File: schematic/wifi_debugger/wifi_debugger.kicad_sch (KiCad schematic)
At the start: 4 parts, among them J1 USB4500-03-0-A_REVA, U1 ESP32-S3-WROOM-1

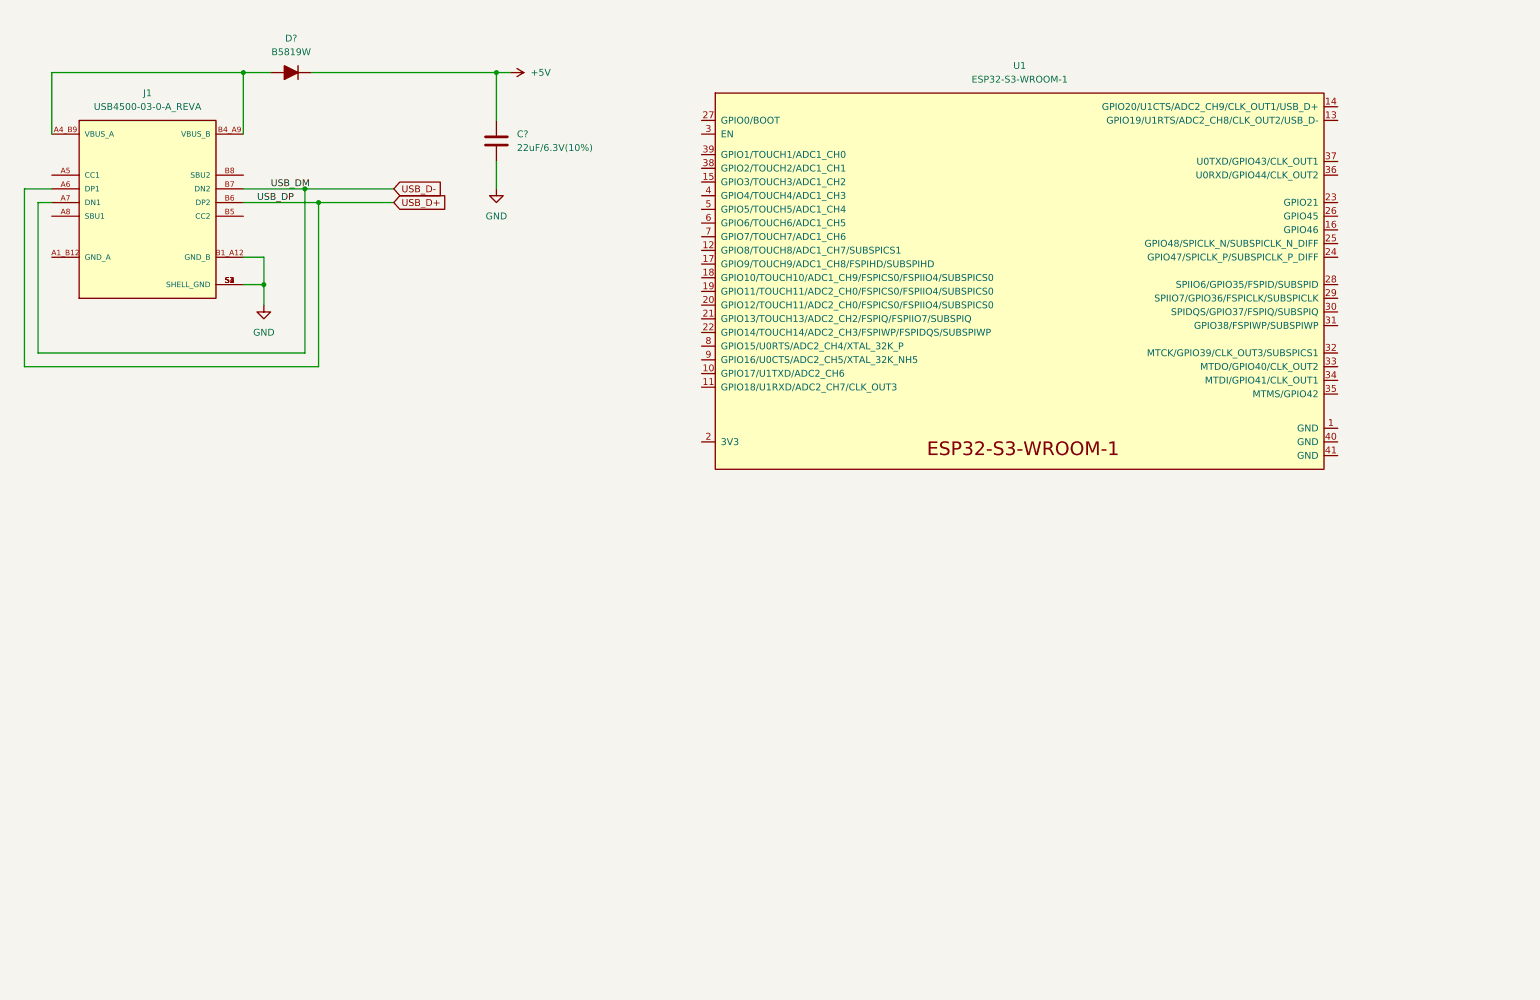
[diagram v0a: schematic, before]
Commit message: update
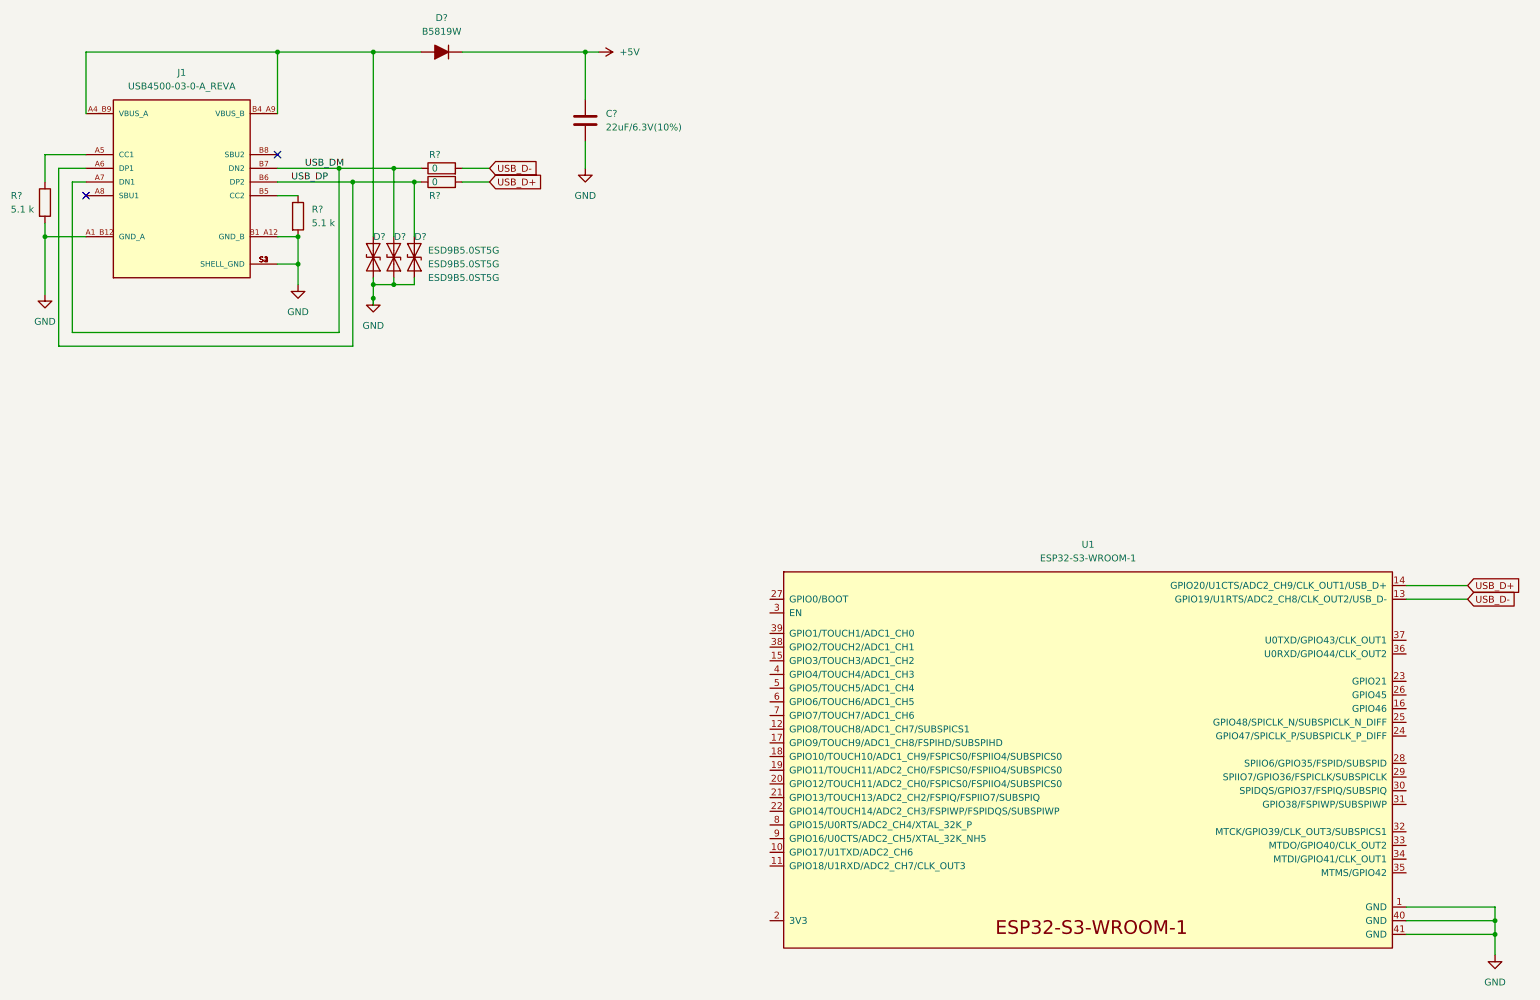
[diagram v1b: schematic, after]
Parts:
- added D? (x3): ESD9B5.0ST5G, Diode_SMD:D_SOD-923, symbol Diode:ESD9B5.0ST5G
- added R? (x2): 5.1 k, symbol Device:R
- added R? (x2): 0, symbol Device:R
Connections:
- net GND: now also J1.A1_B12 (GND_A), U1.1 (GND), U1.40 (GND), U1.41 (GND), D?.1 (A1), D?.1 (A1), D?.1 (A1), R?.2, R?.2
- net USB_D+: now also U1.14 (GPIO20/U1CTS/ADC2_CH9/CLK_OUT1/USB_D+), R?.2; no longer J1.A6 (DP1), J1.B6 (DP2)
- net USB_D-: now also U1.13 (GPIO19/U1RTS/ADC2_CH8/CLK_OUT2/USB_D-), R?.2; no longer J1.A7 (DN1), J1.B7 (DN2)
- net at D?.2 (A), J1.A4_B9 (VBUS_A), J1.B4_A9 (VBUS_B): now also D?.2 (A2)
- net at J1.A5 (CC1): now also R?.1
- net at J1.B5 (CC2): now also R?.1
- new net USB_DM: D?.2 (A2), J1.A7 (DN1), J1.B7 (DN2), R?.1
- new net USB_DP: D?.2 (A2), J1.A6 (DP1), J1.B6 (DP2), R?.1
- no-connect marks 0 -> 2
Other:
- moved on the sheet: C?, D?, J1, U1
